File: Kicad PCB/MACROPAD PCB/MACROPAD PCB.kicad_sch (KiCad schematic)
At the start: 0 parts

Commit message: Schematics
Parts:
- added D1, D10, D11, D12, D13, D14, D15, D16, D2, D3, D4, D5, D6, D7, D8, D9: 1N4148, Diode_THT:D_DO-35_SOD27_P7.62mm_Horizontal, symbol Diode:1N4148
- added SW1, SW10, SW11, SW12, SW13, SW14, SW15, SW16, SW2, SW3, SW4, SW5, SW6, SW7, SW8, SW9: SW_Push, Button_Switch_Keyboard:SW_Cherry_MX_1.00u_Plate, symbol Switch:SW_Push
- added U1: ESP32-S3-MINI-1, RF_Module:ESP32-S2-MINI-1, symbol RF_Module:ESP32-S3-MINI-1
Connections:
- new net: D5.2 (A), SW5.1
- new net: D8.2 (A), SW8.1
- new net: D11.2 (A), SW11.1
- new net: D10.2 (A), SW10.1
- new net: D13.2 (A), SW13.1
- new net: D3.2 (A), SW3.1
- new net: D7.2 (A), SW7.1
- new net: D6.2 (A), SW6.1
- new net: D2.2 (A), SW2.1
- new net: D4.2 (A), SW4.1
- new net: D16.2 (A), SW16.1
- new net: D15.2 (A), SW15.1
- new net: D9.2 (A), SW9.1
- new net: D14.2 (A), SW14.1
- new net: D12.2 (A), SW12.1
- new net: D1.2 (A), SW1.1
- new net COL0: SW1.2, SW13.2, SW5.2, SW9.2, U1.9 (IO5)
- new net COL1: SW10.2, SW14.2, SW2.2, SW6.2, U1.10 (IO6)
- new net COL2: SW11.2, SW15.2, SW3.2, SW7.2, U1.11 (IO7)
- new net COL3: SW12.2, SW16.2, SW4.2, SW8.2, U1.12 (IO8)
- new net GND: U1.1 (GND), U1.2 (GND), U1.42 (GND), U1.43 (GND), U1.46 (GND), U1.47 (GND), U1.48 (GND), U1.49 (GND), U1.50 (GND), U1.51 (GND), U1.52 (GND), U1.53 (GND), U1.54 (GND), U1.55 (GND), U1.56 (GND), U1.57 (GND), U1.58 (GND), U1.59 (GND), U1.60 (GND), U1.61 (GND), U1.62 (GND), U1.63 (GND), U1.64 (GND), U1.65 (GND)
- new net ROW0: D1.1 (K), D2.1 (K), D3.1 (K), D4.1 (K), U1.5 (IO1)
- new net ROW1: D5.1 (K), D6.1 (K), D7.1 (K), D8.1 (K), U1.6 (IO2)
- new net ROW2: D10.1 (K), D11.1 (K), D12.1 (K), D9.1 (K), U1.7 (IO3)
- new net ROW3: D13.1 (K), D14.1 (K), D15.1 (K), D16.1 (K), U1.8 (IO4)

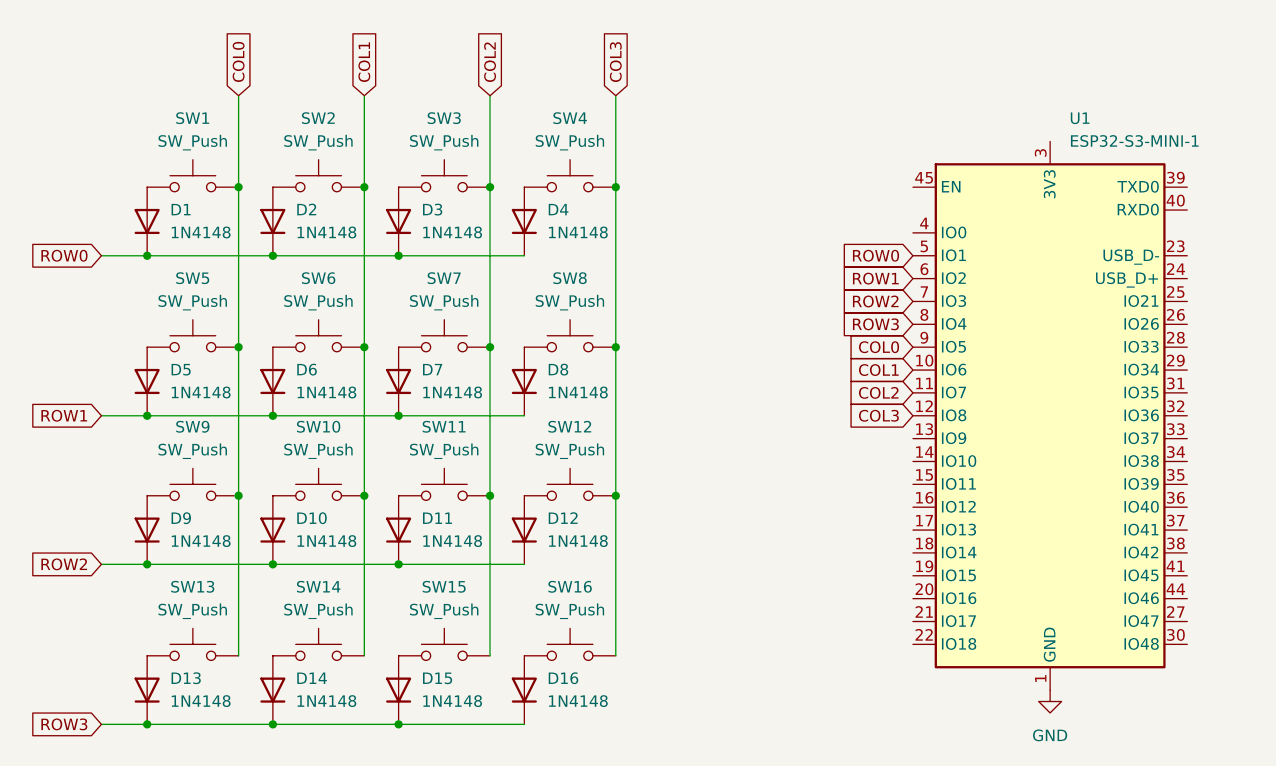
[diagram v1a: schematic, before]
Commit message: pcb
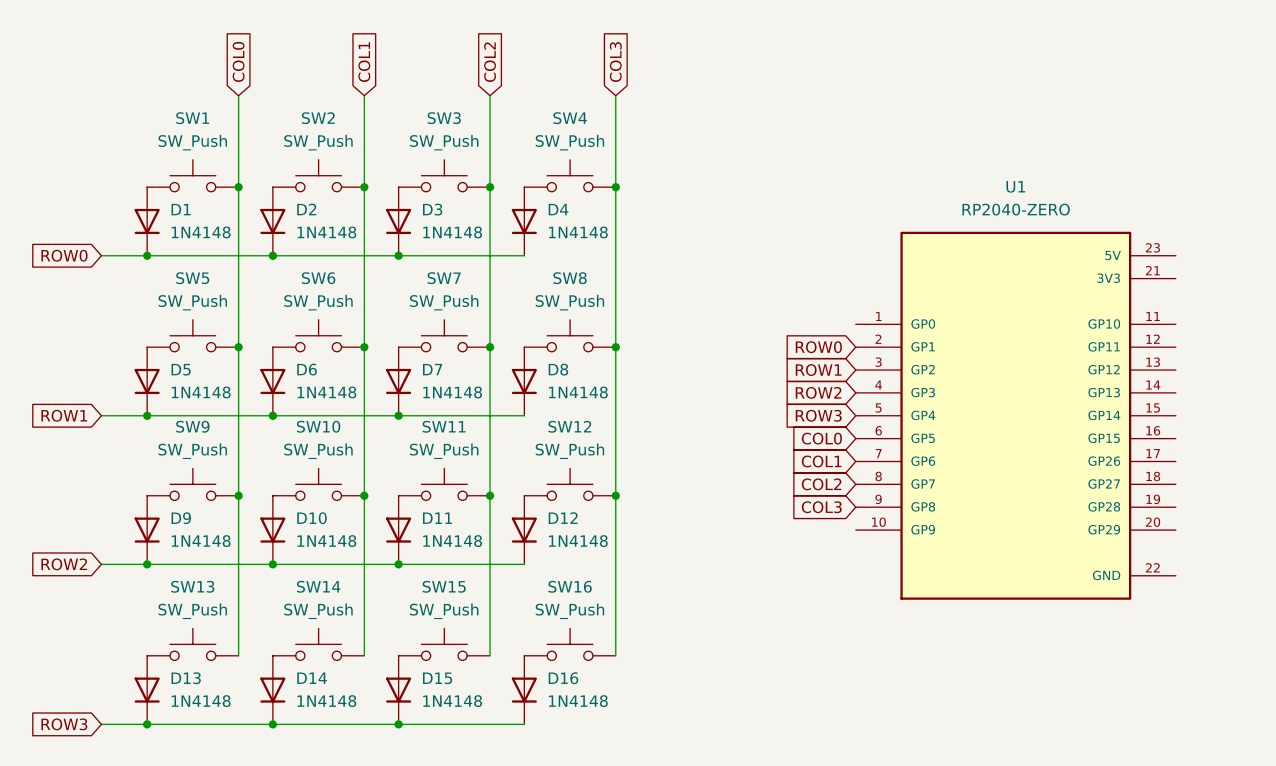
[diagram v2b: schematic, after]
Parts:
- removed U1: ESP32-S3-MINI-1, RF_Module:ESP32-S2-MINI-1, symbol RF_Module:ESP32-S3-MINI-1
- added U1: RP2040-ZERO, RP2040-ZERO:MODULE_RP2040-ZERO, symbol RP2040-ZERO:RP2040-ZERO
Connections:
- net COL0: now also U1.6 (GP5)
- net COL1: now also U1.7 (GP6)
- net COL2: now also U1.8 (GP7)
- net COL3: now also U1.9 (GP8)
- net ROW0: now also U1.2 (GP1)
- net ROW1: now also U1.3 (GP2)
- net ROW2: now also U1.4 (GP3)
- net ROW3: now also U1.5 (GP4)

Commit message: PCB
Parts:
- SW1, SW10, SW11, SW12, SW13, SW14, SW15, SW16, SW2, SW3, SW4, SW5, SW6, SW7, SW8, SW9: footprint Button_Switch_Keyboard:SW_Cherry_MX_1.00u_Plate -> PCM_Switch_Keyboard_Cherry_MX:SW_Cherry_MX_PCB_1.00u
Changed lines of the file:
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@@
 			)
 		)
-		(property "Footprint" "Button_Switch_Keyboard:SW_Cherry_MX_1.00u_Plate"
+		(property "Footprint" "PCM_Switch_Keyboard_Cherry_MX:SW_Cherry_MX_PCB_1.00u"
 			(at 85.09 45.72 0)
 			(hide yes)
@@
 			)
 		)
-		(property "Footprint" "Button_Switch_Keyboard:SW_Cherry_MX_1.00u_Plate"
+		(property "Footprint" "PCM_Switch_Keyboard_Cherry_MX:SW_Cherry_MX_PCB_1.00u"
 			(at 71.12 62.23 0)
 			(hide yes)
@@
 			)
 		)
-		(property "Footprint" "Button_Switch_Keyboard:SW_Cherry_MX_1.00u_Plate"
+		(property "Footprint" "PCM_Switch_Keyboard_Cherry_MX:SW_Cherry_MX_PCB_1.00u"
 			(at 71.12 27.94 0)
 			(hide yes)
@@
 			)
 		)
-		(property "Footprint" "Button_Switch_Keyboard:SW_Cherry_MX_1.00u_Plate"
+		(property "Footprint" "PCM_Switch_Keyboard_Cherry_MX:SW_Cherry_MX_PCB_1.00u"
 			(at 57.15 45.72 0)
 			(hide yes)
@@
 			)
 		)
-		(property "Footprint" "Button_Switch_Keyboard:SW_Cherry_MX_1.00u_Plate"
+		(property "Footprint" "PCM_Switch_Keyboard_Cherry_MX:SW_Cherry_MX_PCB_1.00u"
 			(at 57.15 27.94 0)
 			(hide yes)
@@
 			)
 		)
-		(property "Footprint" "Button_Switch_Keyboard:SW_Cherry_MX_1.00u_Plate"
+		(property "Footprint" "PCM_Switch_Keyboard_Cherry_MX:SW_Cherry_MX_PCB_1.00u"
 			(at 71.12 45.72 0)
 			(hide yes)
@@
 			)
 		)
-		(property "Footprint" "Button_Switch_Keyboard:SW_Cherry_MX_1.00u_Plate"
+		(property "Footprint" "PCM_Switch_Keyboard_Cherry_MX:SW_Cherry_MX_PCB_1.00u"
 			(at 71.12 80.01 0)
 			(hide yes)
@@
 			)
 		)
-		(property "Footprint" "Button_Switch_Keyboard:SW_Cherry_MX_1.00u_Plate"
+		(property "Footprint" "PCM_Switch_Keyboard_Cherry_MX:SW_Cherry_MX_PCB_1.00u"
 			(at 85.09 80.01 0)
 			(hide yes)
@@
 			)
 		)
-		(property "Footprint" "Button_Switch_Keyboard:SW_Cherry_MX_1.00u_Plate"
+		(property "Footprint" "PCM_Switch_Keyboard_Cherry_MX:SW_Cherry_MX_PCB_1.00u"
 			(at 85.09 62.23 0)
 			(hide yes)
@@
 			)
 		)
-		(property "Footprint" "Button_Switch_Keyboard:SW_Cherry_MX_1.00u_Plate"
+		(property "Footprint" "PCM_Switch_Keyboard_Cherry_MX:SW_Cherry_MX_PCB_1.00u"
 			(at 57.15 80.01 0)
 			(hide yes)
@@
 			)
 		)
-		(property "Footprint" "Button_Switch_Keyboard:SW_Cherry_MX_1.00u_Plate"
+		(property "Footprint" "PCM_Switch_Keyboard_Cherry_MX:SW_Cherry_MX_PCB_1.00u"
 			(at 43.18 62.23 0)
 			(hide yes)
@@
 			)
 		)
-		(property "Footprint" "Button_Switch_Keyboard:SW_Cherry_MX_1.00u_Plate"
+		(property "Footprint" "PCM_Switch_Keyboard_Cherry_MX:SW_Cherry_MX_PCB_1.00u"
 			(at 57.15 62.23 0)
 			(hide yes)
@@
 			)
 		)
-		(property "Footprint" "Button_Switch_Keyboard:SW_Cherry_MX_1.00u_Plate"
+		(property "Footprint" "PCM_Switch_Keyboard_Cherry_MX:SW_Cherry_MX_PCB_1.00u"
 			(at 85.09 27.94 0)
 			(hide yes)
@@
 			)
 		)
-		(property "Footprint" "Button_Switch_Keyboard:SW_Cherry_MX_1.00u_Plate"
+		(property "Footprint" "PCM_Switch_Keyboard_Cherry_MX:SW_Cherry_MX_PCB_1.00u"
 			(at 43.18 27.94 0)
 			(hide yes)
@@
 			)
 		)
-		(property "Footprint" "Button_Switch_Keyboard:SW_Cherry_MX_1.00u_Plate"
+		(property "Footprint" "PCM_Switch_Keyboard_Cherry_MX:SW_Cherry_MX_PCB_1.00u"
 			(at 43.18 80.01 0)
 			(hide yes)
@@
 			)
 		)
-		(property "Footprint" "Button_Switch_Keyboard:SW_Cherry_MX_1.00u_Plate"
+		(property "Footprint" "PCM_Switch_Keyboard_Cherry_MX:SW_Cherry_MX_PCB_1.00u"
 			(at 43.18 45.72 0)
 			(hide yes)
